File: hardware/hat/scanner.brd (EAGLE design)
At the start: 65 x 56 mm, 30 parts, among them J1 PJ-102AH, U1 CAT24C32WI-GT3, U2 TPS61165DBV

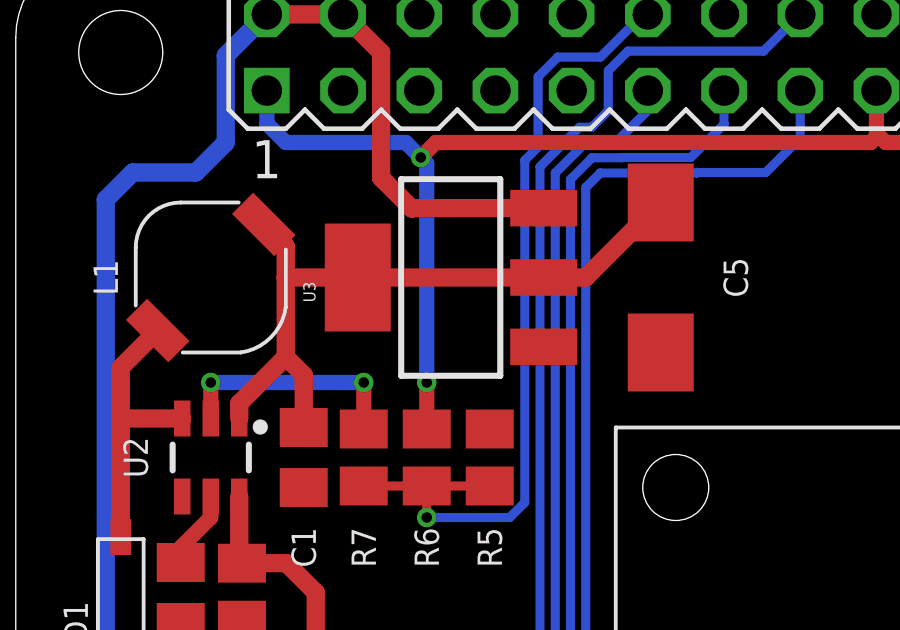
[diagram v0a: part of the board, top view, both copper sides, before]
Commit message: .
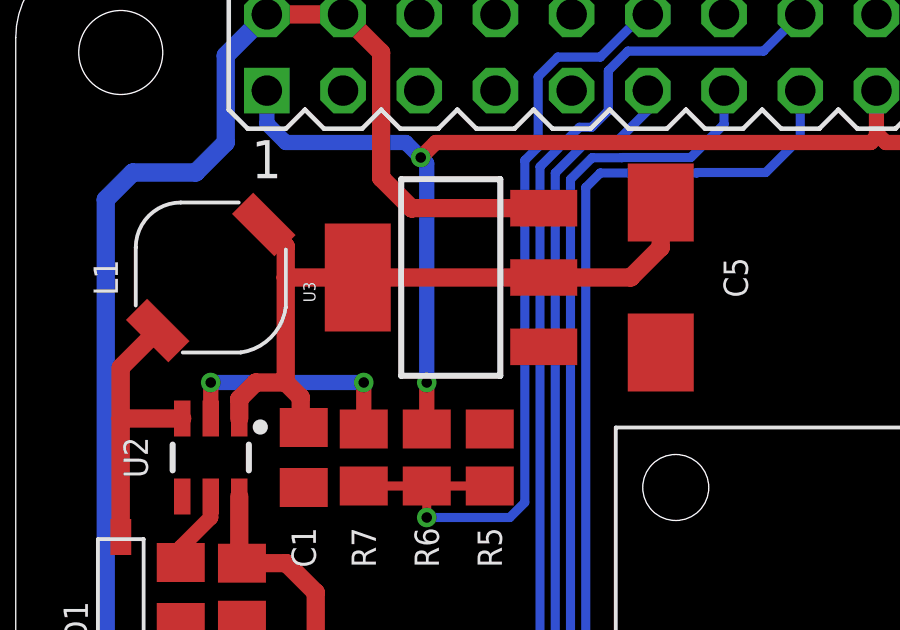
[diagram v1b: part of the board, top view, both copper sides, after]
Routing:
- net VCC: track 23.5 -> 24.2 mm
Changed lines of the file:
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@@
 <contactref element="L1" pad="1"/>
 <wire x1="-23.5" y1="-6.4644625" x2="-24.23223125" y2="-5.73223125" width="0.6096" layer="1"/>
-<wire x1="-23.5" y1="-10.1499" x2="-25.05" y2="-11.6999" width="0.6096" layer="1"/>
-<wire x1="-25.05" y1="-11.6999" x2="-25.05" y2="-12.1999" width="0.6096" layer="1"/>
-<wire x1="-23.5" y1="-10.1499" x2="-23.5" y2="-7.5" width="0.6096" layer="1"/>
 <wire x1="-23.5" y1="-7.5" x2="-23.5" y2="-6.4644625" width="0.6096" layer="1"/>
-<wire x1="-23.5" y1="-10.1499" x2="-22.9" y2="-10.7499" width="0.6096" layer="1"/>
-<wire x1="-22.9" y1="-10.7499" x2="-22.9" y2="-12.5" width="0.6096" layer="1"/>
 <contactref element="U3" pad="4"/>
 <contactref element="U3" pad="2"/>
@@
 <wire x1="-21.099" y1="-7.5" x2="-23.5" y2="-7.5" width="0.6096" layer="1"/>
 <wire x1="-14.9012" y1="-7.5" x2="-21.099" y2="-7.5" width="0.6096" layer="1"/>
-<wire x1="-14.9012" y1="-7.5" x2="-13.5" y2="-7.5" width="0.6096" layer="1"/>
-<wire x1="-13.5" y1="-7.5" x2="-11" y2="-5" width="0.6096" layer="1"/>
+<wire x1="-14.9012" y1="-7.5" x2="-12" y2="-7.5" width="0.6096" layer="1"/>
+<wire x1="-11" y1="-6.5" x2="-11" y2="-5" width="0.6096" layer="1"/>
+<wire x1="-11" y1="-6.5" x2="-12" y2="-7.5" width="0.6096" layer="1"/>
+<wire x1="-22.9" y1="-12.5" x2="-23" y2="-12.4" width="0.6096" layer="1"/>
+<wire x1="-23" y1="-12.4" x2="-23" y2="-11.5" width="0.6096" layer="1"/>
+<wire x1="-23" y1="-11.5" x2="-23.5" y2="-11" width="0.6096" layer="1"/>
+<wire x1="-23.5" y1="-11" x2="-24.5" y2="-11" width="0.6096" layer="1"/>
+<wire x1="-24.5" y1="-11" x2="-25.05" y2="-11.55" width="0.6096" layer="1"/>
+<wire x1="-25.05" y1="-11.55" x2="-25.05" y2="-12.1999" width="0.6096" layer="1"/>
+<wire x1="-23.5" y1="-7.5" x2="-23.5" y2="-11" width="0.6096" layer="1"/>
 </signal>
 </signals>
